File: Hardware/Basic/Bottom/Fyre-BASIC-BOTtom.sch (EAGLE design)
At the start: 38 parts, among them U3 PCF8523, Y2 32.7680kHz

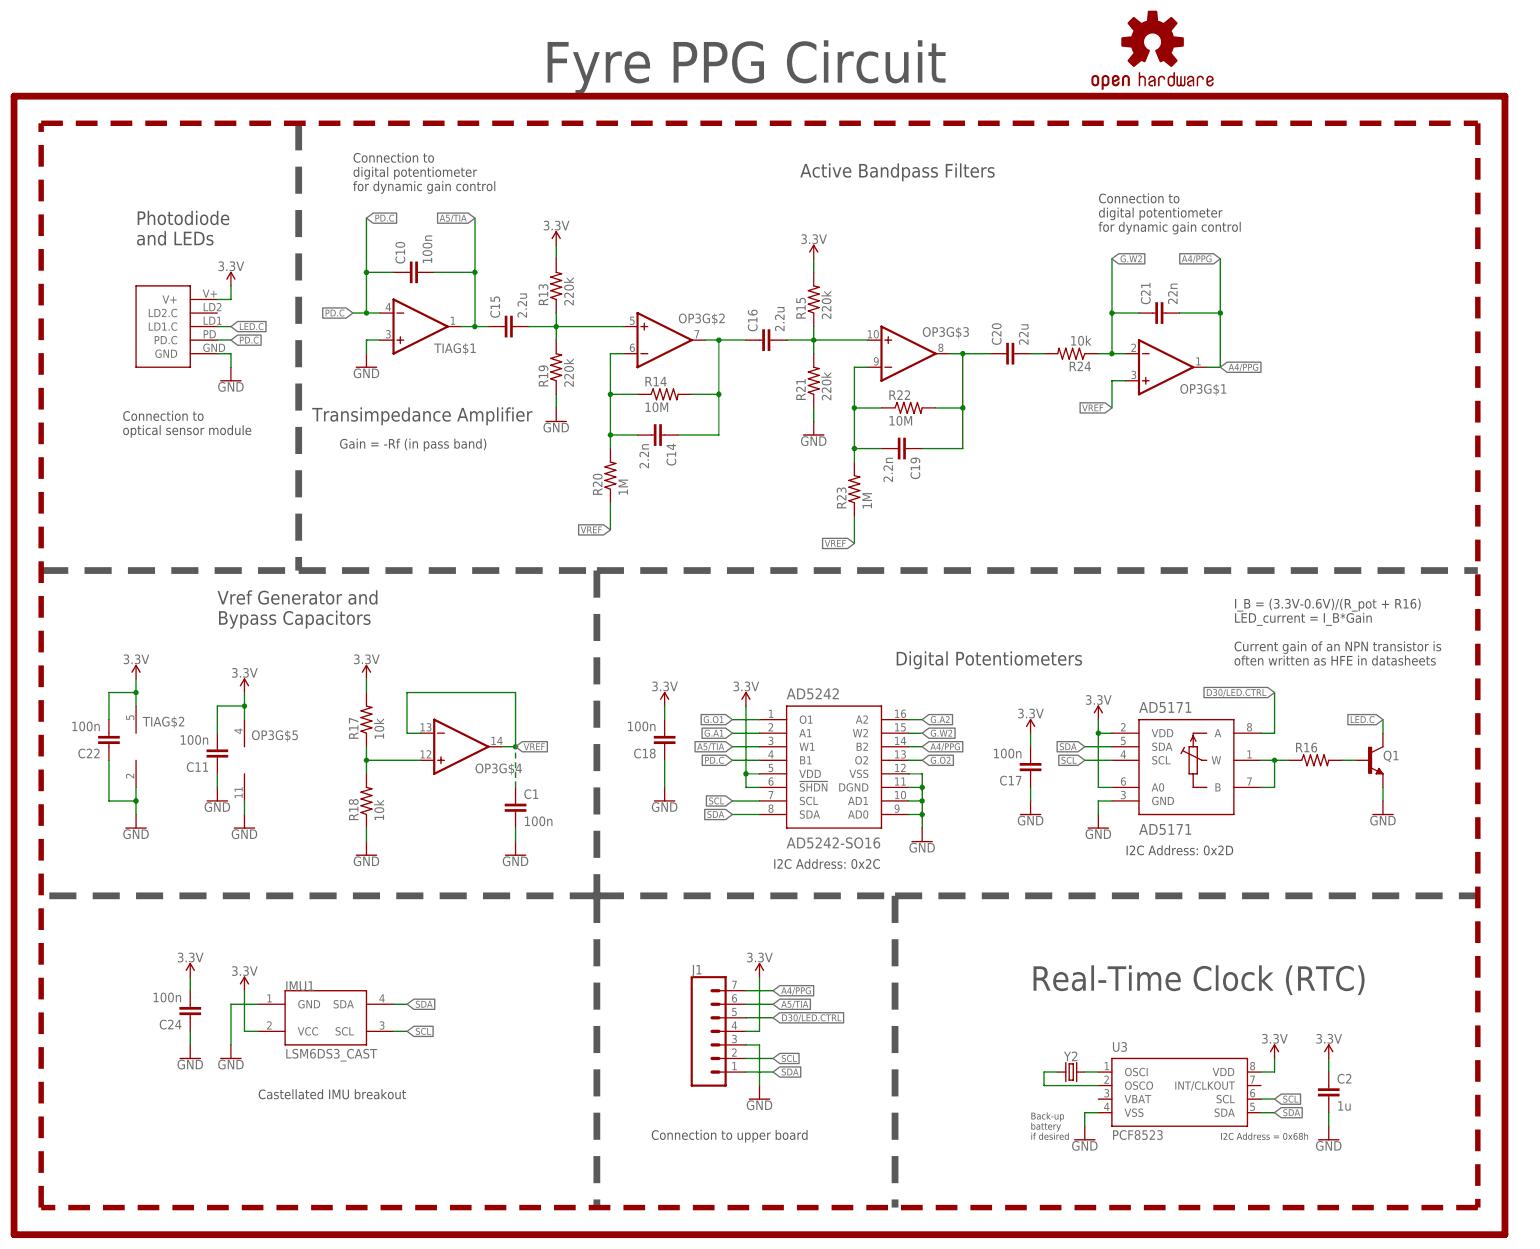
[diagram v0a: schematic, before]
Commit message: Completed the top board
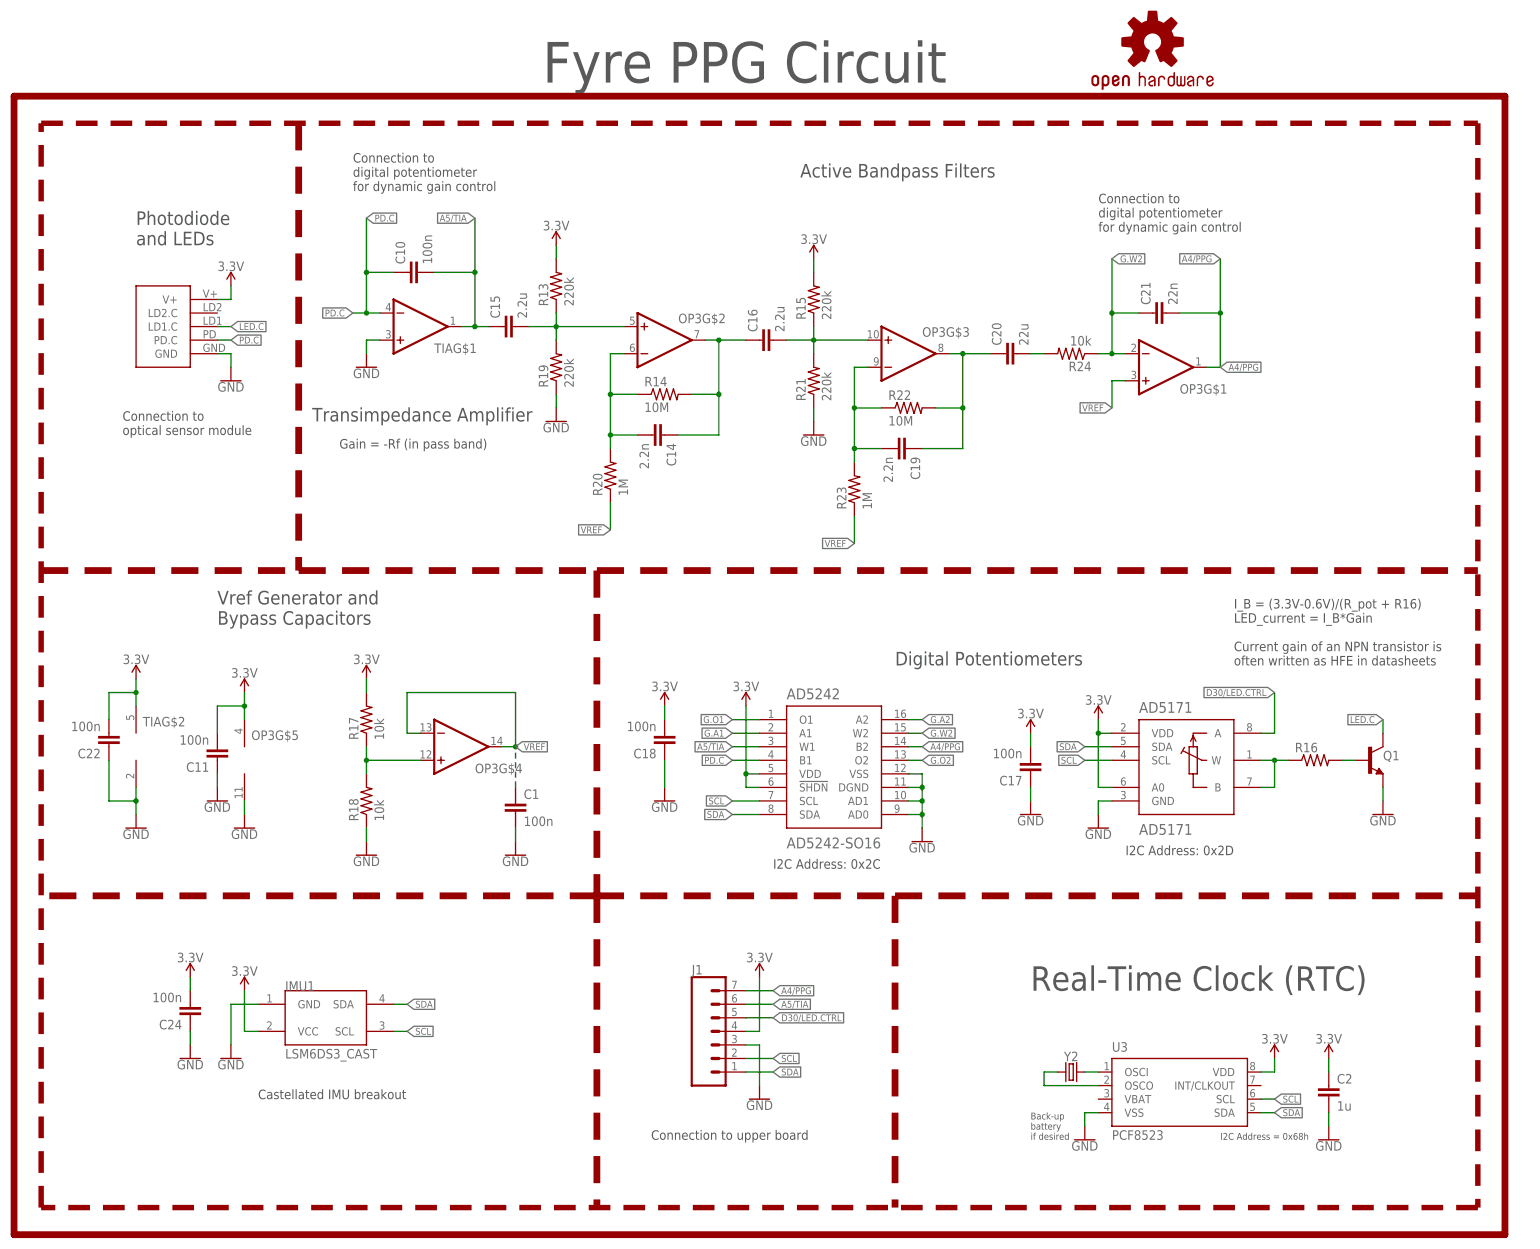
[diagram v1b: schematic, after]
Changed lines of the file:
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@@
 <wire x1="279.4" y1="-30.48" x2="0" y2="-30.48" width="1.27" layer="94"/>
 <wire x1="0" y1="-30.48" x2="0" y2="182.88" width="1.27" layer="94"/>
-<wire x1="5.08" y1="93.98" x2="53.34" y2="93.98" width="1.27" layer="97" style="longdash"/>
-<wire x1="53.34" y1="93.98" x2="109.22" y2="93.98" width="1.27" layer="97" style="longdash"/>
-<wire x1="109.22" y1="93.98" x2="274.32" y2="93.98" width="1.27" layer="97" style="longdash"/>
-<wire x1="109.22" y1="93.98" x2="109.22" y2="33.02" width="1.27" layer="97" style="longdash"/>
-<wire x1="109.22" y1="33.02" x2="109.22" y2="-25.4" width="1.27" layer="97" style="longdash"/>
-<wire x1="109.22" y1="33.02" x2="165.1" y2="33.02" width="1.27" layer="97" style="longdash"/>
-<wire x1="165.1" y1="33.02" x2="274.32" y2="33.02" width="1.27" layer="97" style="longdash"/>
-<wire x1="165.1" y1="33.02" x2="165.1" y2="-25.4" width="1.27" layer="97" style="longdash"/>
-<wire x1="109.22" y1="33.02" x2="5.08" y2="33.02" width="1.27" layer="97" style="longdash"/>
-<wire x1="53.34" y1="177.8" x2="53.34" y2="93.98" width="1.27" layer="97" style="longdash"/>
+<wire x1="5.08" y1="93.98" x2="53.34" y2="93.98" width="1.27" layer="94" style="longdash"/>
+<wire x1="53.34" y1="93.98" x2="109.22" y2="93.98" width="1.27" layer="94" style="longdash"/>
+<wire x1="109.22" y1="93.98" x2="274.32" y2="93.98" width="1.27" layer="94" style="longdash"/>
+<wire x1="109.22" y1="93.98" x2="109.22" y2="33.02" width="1.27" layer="94" style="longdash"/>
+<wire x1="109.22" y1="33.02" x2="109.22" y2="-25.4" width="1.27" layer="94" style="longdash"/>
+<wire x1="109.22" y1="33.02" x2="165.1" y2="33.02" width="1.27" layer="94" style="longdash"/>
+<wire x1="165.1" y1="33.02" x2="274.32" y2="33.02" width="1.27" layer="94" style="longdash"/>
+<wire x1="165.1" y1="33.02" x2="165.1" y2="-25.4" width="1.27" layer="94" style="longdash"/>
+<wire x1="109.22" y1="33.02" x2="5.08" y2="33.02" width="1.27" layer="94" style="longdash"/>
+<wire x1="53.34" y1="177.8" x2="53.34" y2="93.98" width="1.27" layer="94" style="longdash"/>
 <text x="20.32" y="119.38" size="1.778" layer="97">Connection to
 optical sensor module</text>
